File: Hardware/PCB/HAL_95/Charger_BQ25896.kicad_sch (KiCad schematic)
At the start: 52 parts, among them J9 Battery, Q1 DMN313DLT-7, Q2 DMP1045U-7, Q3 MMDT2907A-7-F, SW3 nQON, U3 BU33SD5WG-TR, U5 BQ25896RTW, U8 BQ27220YZFR

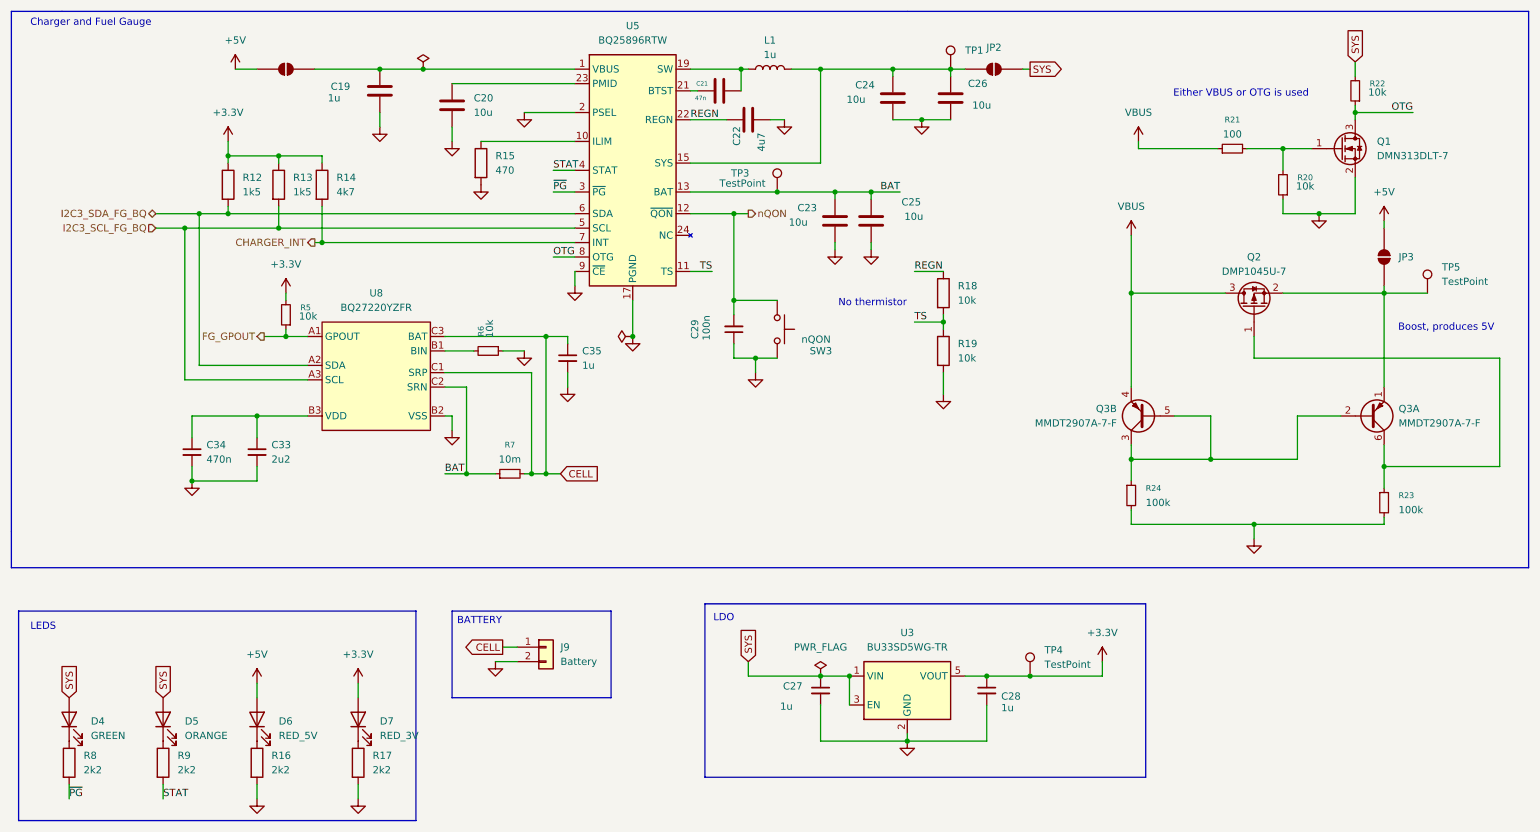
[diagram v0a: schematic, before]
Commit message: removed erc errors
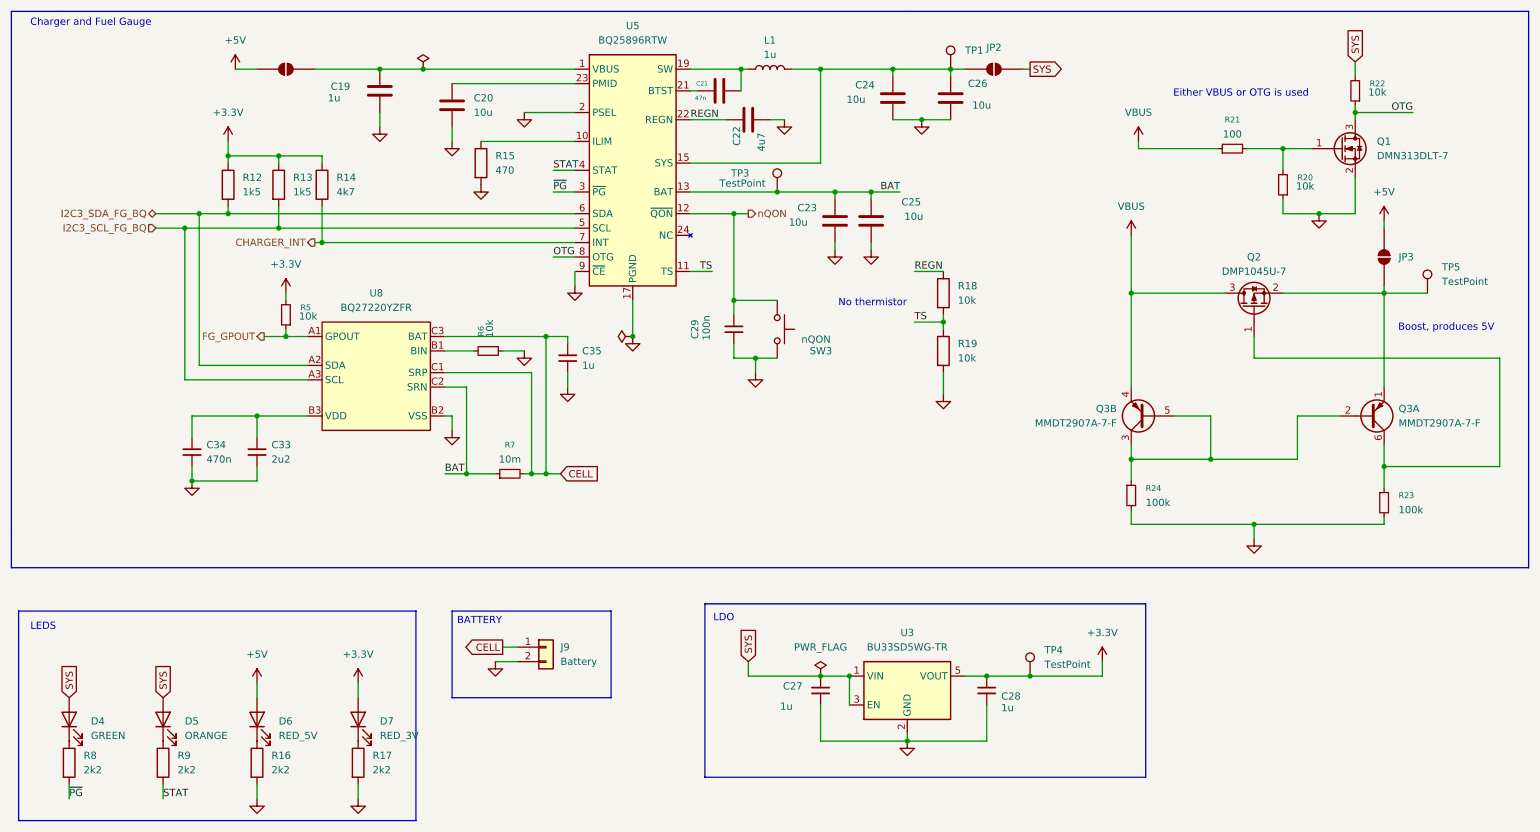
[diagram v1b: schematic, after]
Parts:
- JP1, JP2, JP3: footprint (none) -> Jumper:SolderJumper-2_P1.3mm_Open_TrianglePad1.0x1.5mm
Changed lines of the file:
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@@
 			)
 		)
-		(property "Footprint" ""
+		(property "Footprint" "Jumper:SolderJumper-2_P1.3mm_Open_TrianglePad1.0x1.5mm"
 			(at 255.27 62.23 0)
 			(hide yes)
@@
 			)
 		)
-		(property "Footprint" ""
+		(property "Footprint" "Jumper:SolderJumper-2_P1.3mm_Open_TrianglePad1.0x1.5mm"
 			(at 62.23 29.21 0)
 			(hide yes)
@@
 			)
 		)
-		(property "Footprint" ""
+		(property "Footprint" "Jumper:SolderJumper-2_P1.3mm_Open_TrianglePad1.0x1.5mm"
 			(at 186.69 29.21 0)
 			(hide yes)
